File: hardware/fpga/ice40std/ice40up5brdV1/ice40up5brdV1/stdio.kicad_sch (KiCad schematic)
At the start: 17 parts, among them J1 Conn_01x20_Male, J2 Conn_01x20_Female

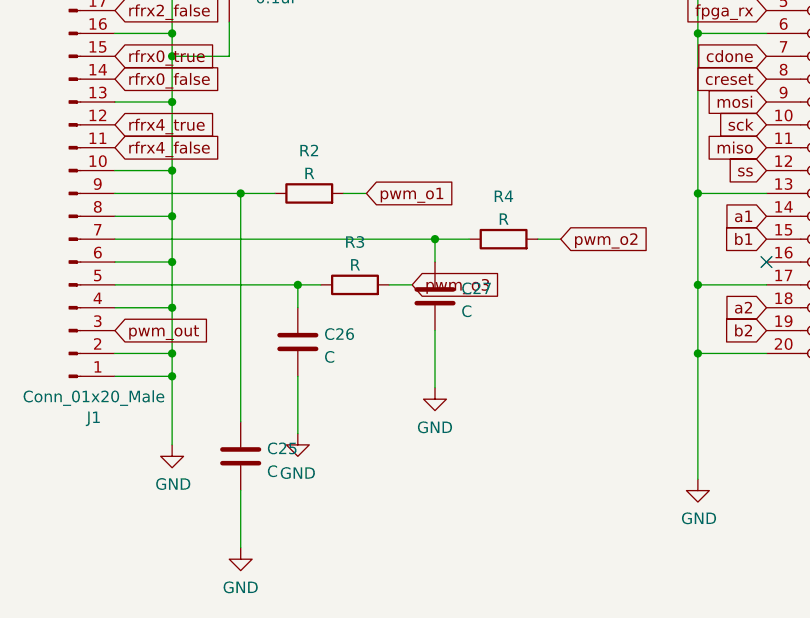
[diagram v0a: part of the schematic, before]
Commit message: pwm / lvds power / filters
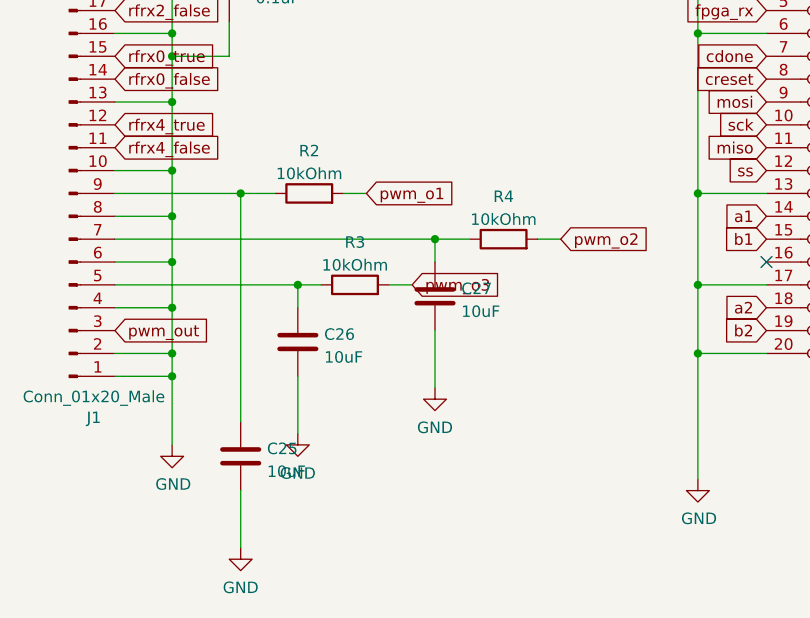
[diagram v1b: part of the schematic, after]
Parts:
- C25, C26, C27: value C -> 10uF; footprint (none) -> Capacitor_SMD:C_1206_3216Metric
- R2, R3, R4: value R -> 10kOhm; footprint (none) -> Resistor_SMD:R_1206_3216Metric
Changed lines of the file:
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@@
     (in_bom yes) (on_board yes) (fields_autoplaced)
     (property "Reference" "R3" (id 0) (at 93.98 87.9942 90))
-    (property "Value" "R" (id 1) (at 93.98 90.5311 90))
-    (property "Footprint" "" (id 2) (at 93.98 94.488 90)
+    (property "Value" "10kOhm" (id 1) (at 93.98 90.5311 90))
+    (property "Footprint" "Resistor_SMD:R_1206_3216Metric" (id 2) (at 93.98 94.488 90)
       (effects (font (size 1.27 1.27)) hide)
     )
@@
       (effects (font (size 1.27 1.27)) (justify left))
     )
-    (property "Value" "C" (id 1) (at 90.551 100.7622 0)
+    (property "Value" "10uF" (id 1) (at 90.551 100.7622 0)
       (effects (font (size 1.27 1.27)) (justify left))
     )
-    (property "Footprint" "" (id 2) (at 88.5952 102.87 0)
+    (property "Footprint" "Capacitor_SMD:C_1206_3216Metric" (id 2) (at 88.5952 102.87 0)
       (effects (font (size 1.27 1.27)) hide)
     )
@@
       (effects (font (size 1.27 1.27)) (justify left))
     )
-    (property "Value" "C" (id 1) (at 84.201 113.4622 0)
+    (property "Value" "10uF" (id 1) (at 84.201 113.4622 0)
       (effects (font (size 1.27 1.27)) (justify left))
     )
-    (property "Footprint" "" (id 2) (at 82.2452 115.57 0)
+    (property "Footprint" "Capacitor_SMD:C_1206_3216Metric" (id 2) (at 82.2452 115.57 0)
       (effects (font (size 1.27 1.27)) hide)
     )
@@
       (effects (font (size 1.27 1.27)) (justify left))
     )
-    (property "Value" "C" (id 1) (at 105.791 95.6822 0)
+    (property "Value" "10uF" (id 1) (at 105.791 95.6822 0)
       (effects (font (size 1.27 1.27)) (justify left))
     )
-    (property "Footprint" "" (id 2) (at 103.8352 97.79 0)
+    (property "Footprint" "Capacitor_SMD:C_1206_3216Metric" (id 2) (at 103.8352 97.79 0)
       (effects (font (size 1.27 1.27)) hide)
     )
@@
     (in_bom yes) (on_board yes) (fields_autoplaced)
     (property "Reference" "R4" (id 0) (at 110.49 82.9142 90))
-    (property "Value" "R" (id 1) (at 110.49 85.4511 90))
-    (property "Footprint" "" (id 2) (at 110.49 89.408 90)
+    (property "Value" "10kOhm" (id 1) (at 110.49 85.4511 90))
+    (property "Footprint" "Resistor_SMD:R_1206_3216Metric" (id 2) (at 110.49 89.408 90)
       (effects (font (size 1.27 1.27)) hide)
     )
@@
     (in_bom yes) (on_board yes) (fields_autoplaced)
     (property "Reference" "R2" (id 0) (at 88.9 77.8342 90))
-    (property "Value" "R" (id 1) (at 88.9 80.3711 90))
-    (property "Footprint" "" (id 2) (at 88.9 84.328 90)
+    (property "Value" "10kOhm" (id 1) (at 88.9 80.3711 90))
+    (property "Footprint" "Resistor_SMD:R_1206_3216Metric" (id 2) (at 88.9 84.328 90)
       (effects (font (size 1.27 1.27)) hide)
     )

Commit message: pwm / lvds power / filters
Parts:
- C25, C26, C27: footprint Capacitor_SMD:C_1206_3216Metric -> Capacitor_SMD:C_0603_1608Metric
- R2, R3, R4: footprint Resistor_SMD:R_1206_3216Metric -> Resistor_SMD:R_0402_1005Metric
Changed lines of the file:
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@@
     (property "Reference" "R3" (id 0) (at 93.98 87.9942 90))
     (property "Value" "10kOhm" (id 1) (at 93.98 90.5311 90))
-    (property "Footprint" "Resistor_SMD:R_1206_3216Metric" (id 2) (at 93.98 94.488 90)
+    (property "Footprint" "Resistor_SMD:R_0402_1005Metric" (id 2) (at 93.98 94.488 90)
       (effects (font (size 1.27 1.27)) hide)
     )
@@
       (effects (font (size 1.27 1.27)) (justify left))
     )
-    (property "Footprint" "Capacitor_SMD:C_1206_3216Metric" (id 2) (at 88.5952 102.87 0)
+    (property "Footprint" "Capacitor_SMD:C_0603_1608Metric" (id 2) (at 88.5952 102.87 0)
       (effects (font (size 1.27 1.27)) hide)
     )
@@
       (effects (font (size 1.27 1.27)) (justify left))
     )
-    (property "Footprint" "Capacitor_SMD:C_1206_3216Metric" (id 2) (at 82.2452 115.57 0)
+    (property "Footprint" "Capacitor_SMD:C_0603_1608Metric" (id 2) (at 82.2452 115.57 0)
       (effects (font (size 1.27 1.27)) hide)
     )
@@
       (effects (font (size 1.27 1.27)) (justify left))
     )
-    (property "Footprint" "Capacitor_SMD:C_1206_3216Metric" (id 2) (at 103.8352 97.79 0)
+    (property "Footprint" "Capacitor_SMD:C_0603_1608Metric" (id 2) (at 103.8352 97.79 0)
       (effects (font (size 1.27 1.27)) hide)
     )
@@
     (property "Reference" "R4" (id 0) (at 110.49 82.9142 90))
     (property "Value" "10kOhm" (id 1) (at 110.49 85.4511 90))
-    (property "Footprint" "Resistor_SMD:R_1206_3216Metric" (id 2) (at 110.49 89.408 90)
+    (property "Footprint" "Resistor_SMD:R_0402_1005Metric" (id 2) (at 110.49 89.408 90)
       (effects (font (size 1.27 1.27)) hide)
     )
@@
     (property "Reference" "R2" (id 0) (at 88.9 77.8342 90))
     (property "Value" "10kOhm" (id 1) (at 88.9 80.3711 90))
-    (property "Footprint" "Resistor_SMD:R_1206_3216Metric" (id 2) (at 88.9 84.328 90)
+    (property "Footprint" "Resistor_SMD:R_0402_1005Metric" (id 2) (at 88.9 84.328 90)
       (effects (font (size 1.27 1.27)) hide)
     )

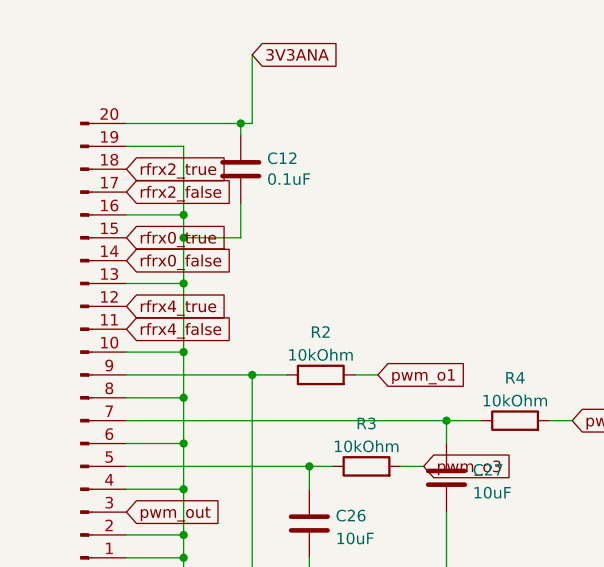
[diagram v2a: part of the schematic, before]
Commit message: pwm / lvds power / filters
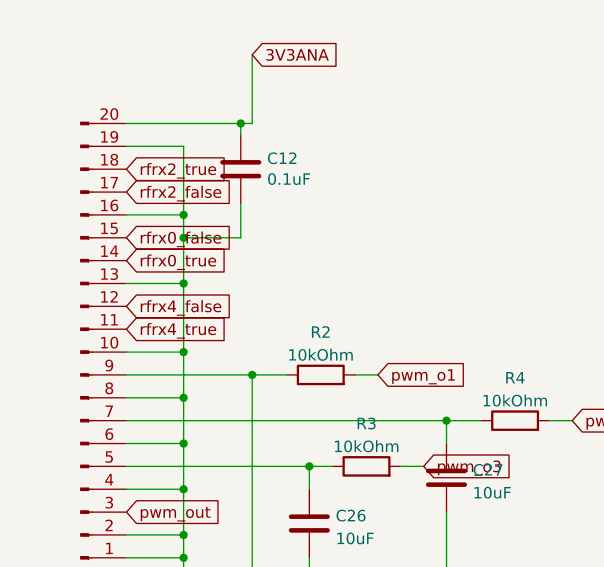
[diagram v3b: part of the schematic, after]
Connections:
- net rfrx0_false: now also J1.15 (Pin_15); no longer J1.14 (Pin_14)
- net rfrx0_true: now also J1.14 (Pin_14); no longer J1.15 (Pin_15)
- net rfrx4_false: now also J1.12 (Pin_12); no longer J1.11 (Pin_11)
- net rfrx4_true: now also J1.11 (Pin_11); no longer J1.12 (Pin_12)
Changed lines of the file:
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@@
     )
   )
-  (global_label "rfrx0_true" (shape input) (at 67.31 67.31 0) (fields_autoplaced)
+  (global_label "rfrx0_true" (shape input) (at 67.31 69.85 0) (fields_autoplaced)
     (effects (font (size 1.27 1.27)) (justify left))
-    (property "Intersheet References" "${INTERSHEET_REFS}" (id 0) (at 0 -7.62 0)
+    (property "Intersheet References" "${INTERSHEET_REFS}" (id 0) (at 0 -5.08 0)
       (effects (font (size 1.27 1.27)) hide)
     )
@@
     )
   )
-  (global_label "rfrx0_false" (shape input) (at 67.31 69.85 0) (fields_autoplaced)
+  (global_label "rfrx0_false" (shape input) (at 67.31 67.31 0) (fields_autoplaced)
     (effects (font (size 1.27 1.27)) (justify left))
-    (property "Intersheet References" "${INTERSHEET_REFS}" (id 0) (at 0 0 0)
+    (property "Intersheet References" "${INTERSHEET_REFS}" (id 0) (at 0 -2.54 0)
       (effects (font (size 1.27 1.27)) hide)
     )
@@
     )
   )
-  (global_label "rfrx4_true" (shape input) (at 67.31 74.93 0) (fields_autoplaced)
+  (global_label "rfrx4_true" (shape input) (at 67.31 77.47 0) (fields_autoplaced)
     (effects (font (size 1.27 1.27)) (justify left))
-    (property "Intersheet References" "${INTERSHEET_REFS}" (id 0) (at 0 -15.24 0)
+    (property "Intersheet References" "${INTERSHEET_REFS}" (id 0) (at 0 -12.7 0)
       (effects (font (size 1.27 1.27)) hide)
     )
@@
     )
   )
-  (global_label "rfrx4_false" (shape input) (at 67.31 77.47 0) (fields_autoplaced)
+  (global_label "rfrx4_false" (shape input) (at 67.31 74.93 0) (fields_autoplaced)
     (effects (font (size 1.27 1.27)) (justify left))
-    (property "Intersheet References" "${INTERSHEET_REFS}" (id 0) (at 0 0 0)
+    (property "Intersheet References" "${INTERSHEET_REFS}" (id 0) (at 0 -2.54 0)
       (effects (font (size 1.27 1.27)) hide)
     )
